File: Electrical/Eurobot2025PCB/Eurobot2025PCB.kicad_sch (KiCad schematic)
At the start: 25 parts, among them J1 Screw_Terminal_01x02, J2 Conn_01x04_Socket, J3 Conn_01x04_Socket, J4 Conn_01x04_Socket, J5 Conn_01x02_Socket, J6 Conn_01x04_Socket, SW2 SW_SPDT, SW3 SW_Push, SW4 SW_Push, U1 INA219, U2 GC9A01, U3 PCA9685, U4 L9110, U5 VL6180X, U6 VL6180X, U7 4R7

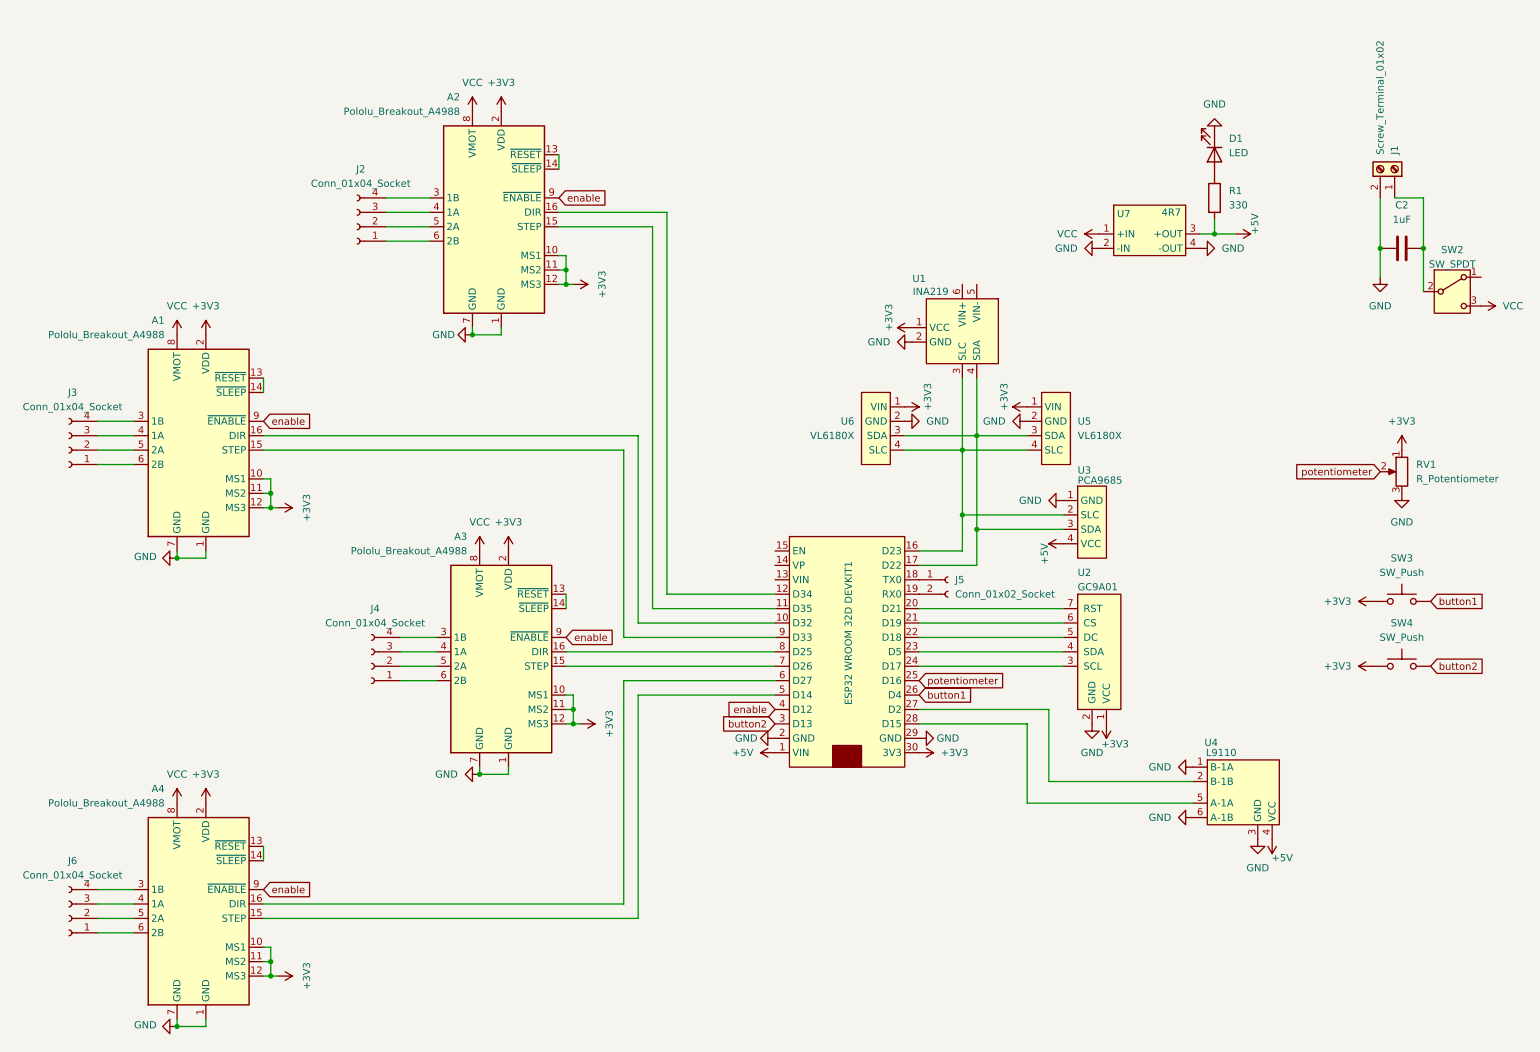
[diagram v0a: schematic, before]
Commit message: update pcb :alien:
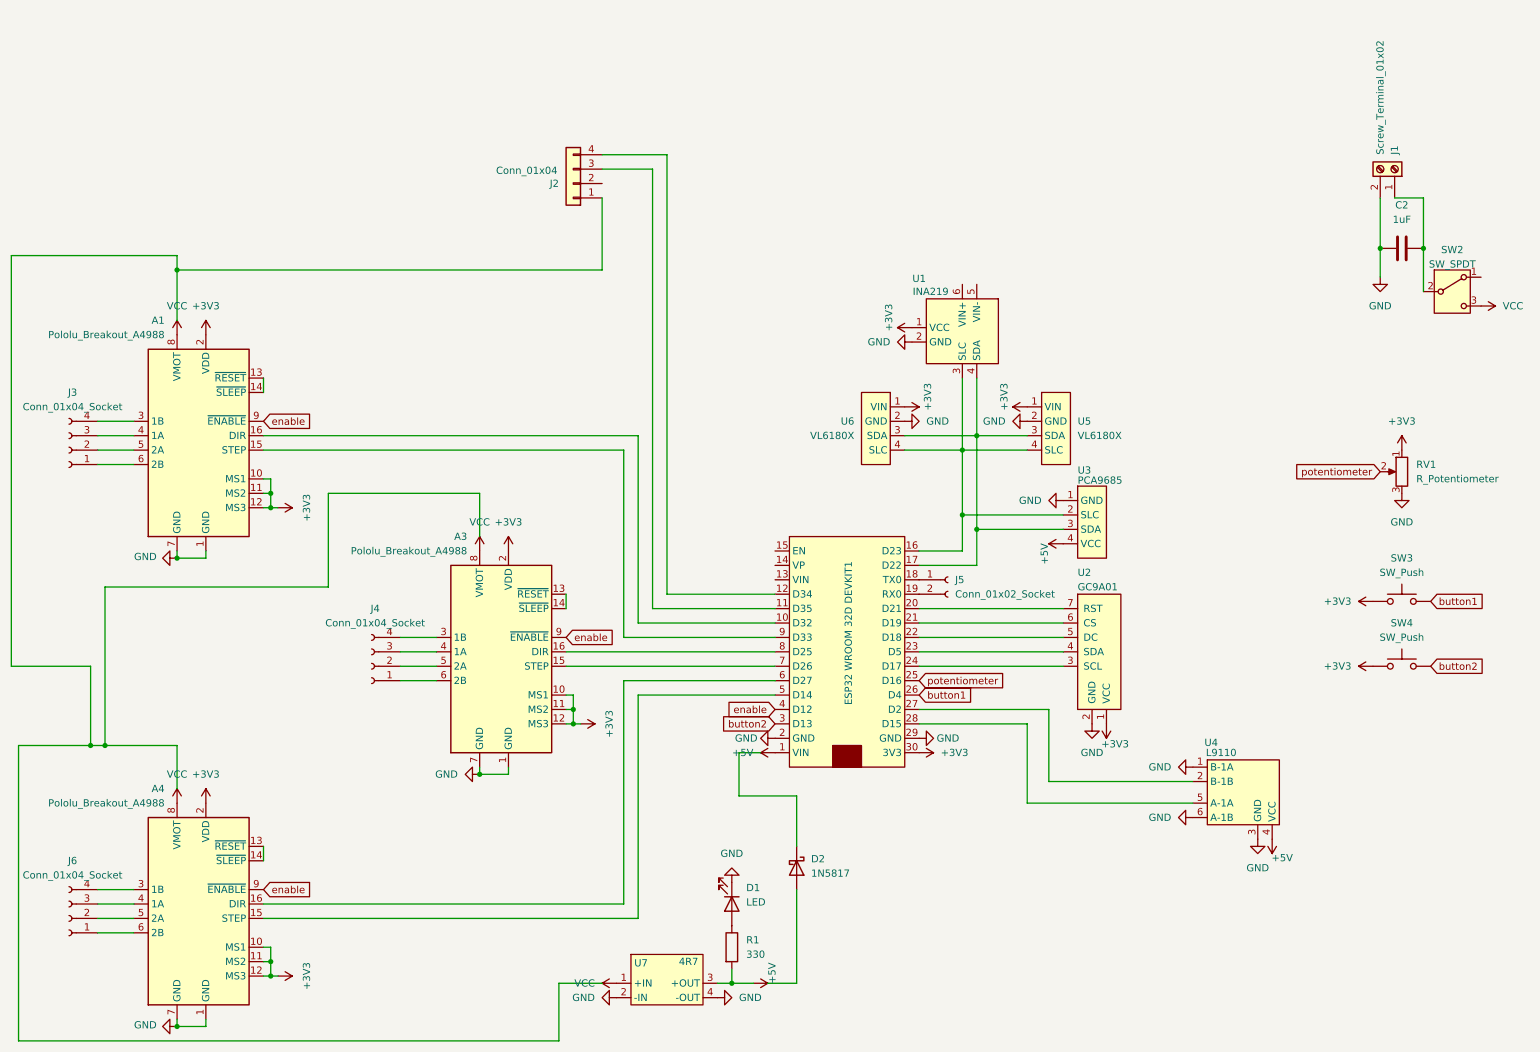
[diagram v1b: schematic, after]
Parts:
- removed A2: Pololu_Breakout_A4988, ECN:A4988, symbol Driver_Motor:Pololu_Breakout_A4988
- removed J2: Conn_01x04_Socket, Connector_JST:JST_XH_B4B-XH-A_1x04_P2.50mm_Vertical, symbol Connector:Conn_01x04_Socket
- added D2: 1N5817, Diode_THT:D_DO-41_SOD81_P10.16mm_Horizontal, symbol Diode:1N5817
- added J2: Conn_01x04, symbol Connector_Generic:Conn_01x04
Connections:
- net at ESP32 WROOM 32D DEVKIT1.11 (D35): now also J2.3 (Pin_3)
- net at ESP32 WROOM 32D DEVKIT1.12 (D34): now also J2.4 (Pin_4)
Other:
- moved on the sheet: D1, R1, U7
